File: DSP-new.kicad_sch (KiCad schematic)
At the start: 16 parts, among them J11 LCD, Q6 AO3400A, SW2 Frequency, SW3 Menu, U6 ESP32-A1S

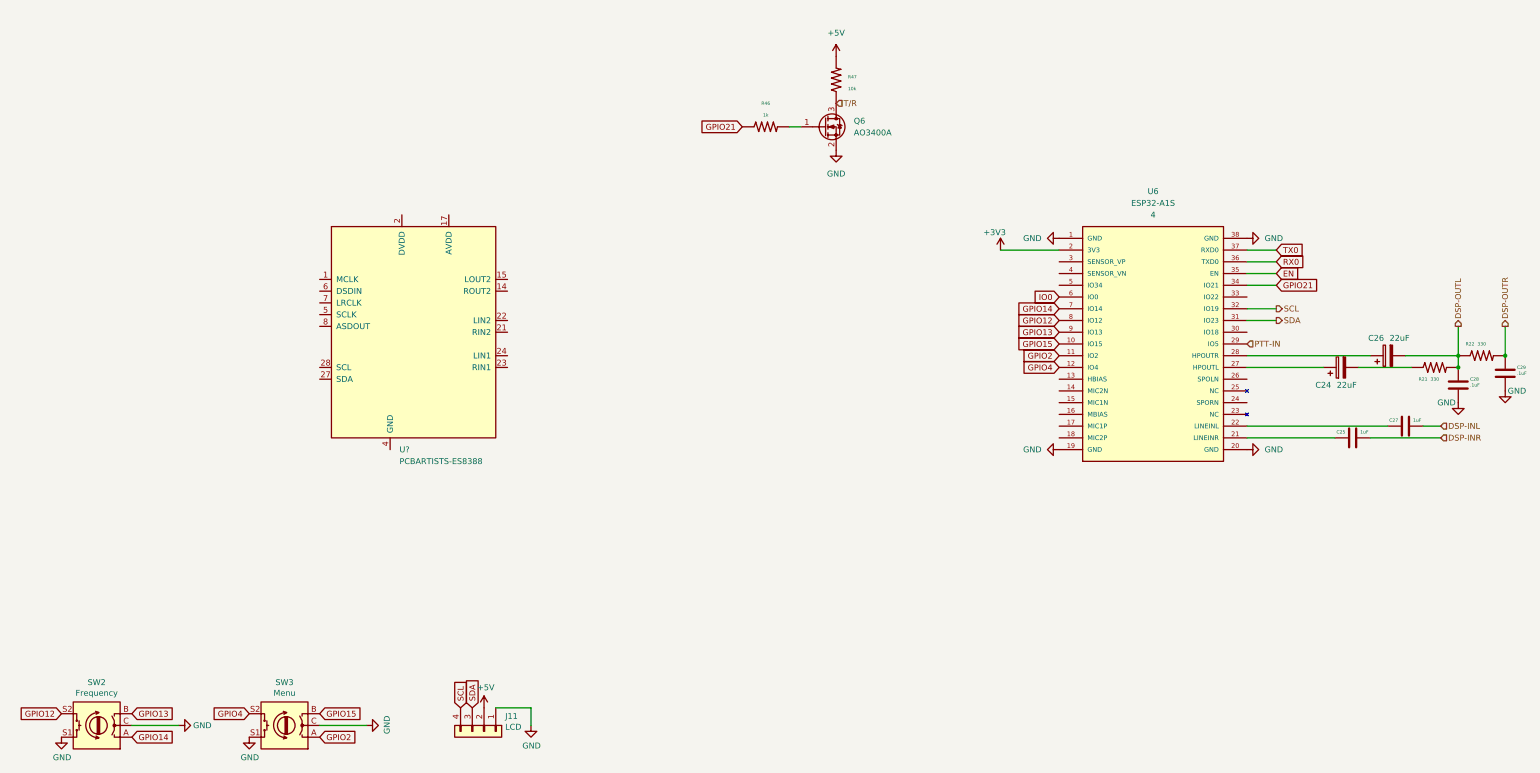
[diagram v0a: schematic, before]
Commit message: added esp32-s3
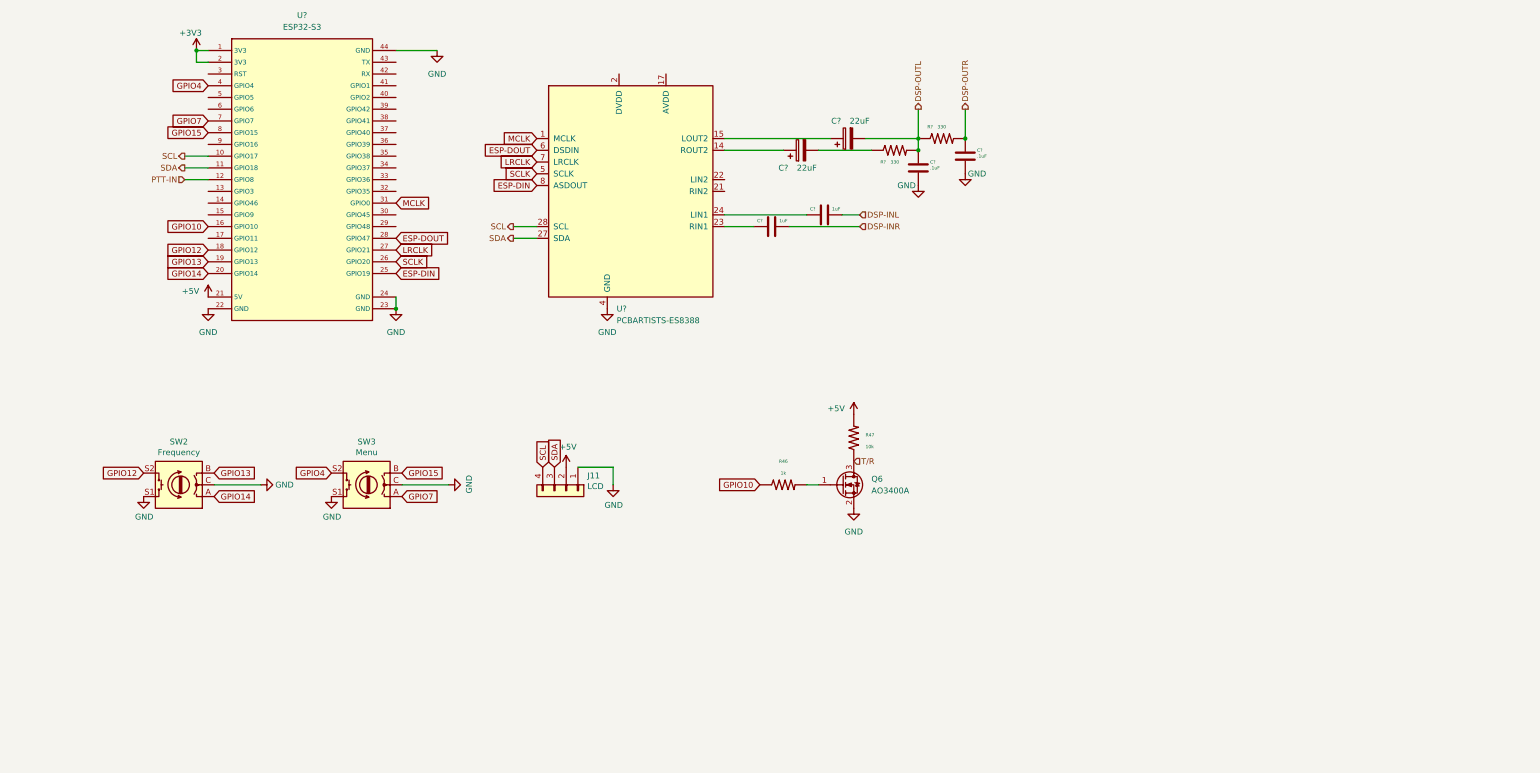
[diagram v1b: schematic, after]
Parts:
- removed C24, C26: 22uF, Capacitor_SMD:CP_Elec_4x4.5, symbol Device:C_Polarized
- removed C25, C27: 1uF, Capacitor_SMD:C_1206_3216Metric, symbol Xenir:Capacitor
- removed C28, C29: .1uF, Capacitor_SMD:C_1206_3216Metric, symbol Xenir:Capacitor
- removed R21, R22: 330, Resistor_SMD:R_0805_2012Metric, symbol Xenir:Resistor
- removed U6: ESP32-A1S, xenir_v6:esp32-a1s-header, symbol Xenir:ESP32-A1S
- added C? (x2): .1uF, Capacitor_SMD:C_1206_3216Metric, symbol Xenir:Capacitor
- added C? (x2): 1uF, Capacitor_SMD:C_1206_3216Metric, symbol Xenir:Capacitor
- added C? (x2): 22uF, Capacitor_SMD:CP_Elec_4x4.5, symbol Device:C_Polarized
- added R? (x2): 330, Resistor_SMD:R_0805_2012Metric, symbol Xenir:Resistor
- added U?: ESP32-S3, symbol xenir_v6:ESP32-S3
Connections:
- net +3V3: now also U?.1 (3V3), U?.2 (3V3)
- net +5V: now also U?.21 (5V)
- net DSP-INL: now also C?.2
- net DSP-INR: now also C?.2
- net DSP-OUTL: now also C?.2, C?.2, R?.1, R?.2
- net DSP-OUTR: now also C?.2, R?.2
- net GND: now also U?.4 (GND), C?.1, C?.1, U?.22 (GND), U?.23 (GND), U?.24 (GND), U?.44 (GND)
- net GPIO12: now also U?.18 (GPIO12)
- net GPIO13: now also U?.19 (GPIO13)
- net GPIO14: now also U?.20 (GPIO14)
- net GPIO15: now also U?.8 (GPIO15)
- net GPIO4: now also U?.4 (GPIO4)
- net PTT-IN: now also U?.12 (GPIO8)
- net SCL: now also U?.28 (SCL), U?.10 (GPIO17)
- net SDA: now also U?.27 (SDA), U?.11 (GPIO18)
- net MCLK: now reaches U?.1 (MCLK)
- net MCLK: now also U?.31 (GPIO0)
- net at U?.14 (ROUT2): now also C?.1
- net at U?.15 (LOUT2): now also C?.1
- net at U?.23 (RIN1): now also C?.1
- net at U?.24 (LIN1): now also C?.1
- net SCLK: now reaches U?.5 (SCLK)
- net SCLK: now also U?.26 (GPIO20)
- net ESP-DOUT: now reaches U?.6 (DSDIN)
- net ESP-DOUT: now also U?.28 (GPIO47)
- net LRCLK: now reaches U?.7 (LRCLK)
- net LRCLK: now also U?.27 (GPIO21)
- net ESP-DIN: now reaches U?.8 (ASDOUT)
- net ESP-DIN: now also U?.25 (GPIO19)
- net GPIO2 renamed GPIO7
- net GPIO7: now also U?.7 (GPIO7)
- net GPIO21 renamed GPIO10
- net GPIO10: now also U?.16 (GPIO10)
- new net: C?.2, R?.1
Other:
- moved on the sheet: J11, Q6, R46, R47, SW2, SW3, U?
